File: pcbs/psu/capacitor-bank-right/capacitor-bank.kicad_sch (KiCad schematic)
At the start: 19 parts, among them J1 Conn_01x03, J2 Conn_01x03

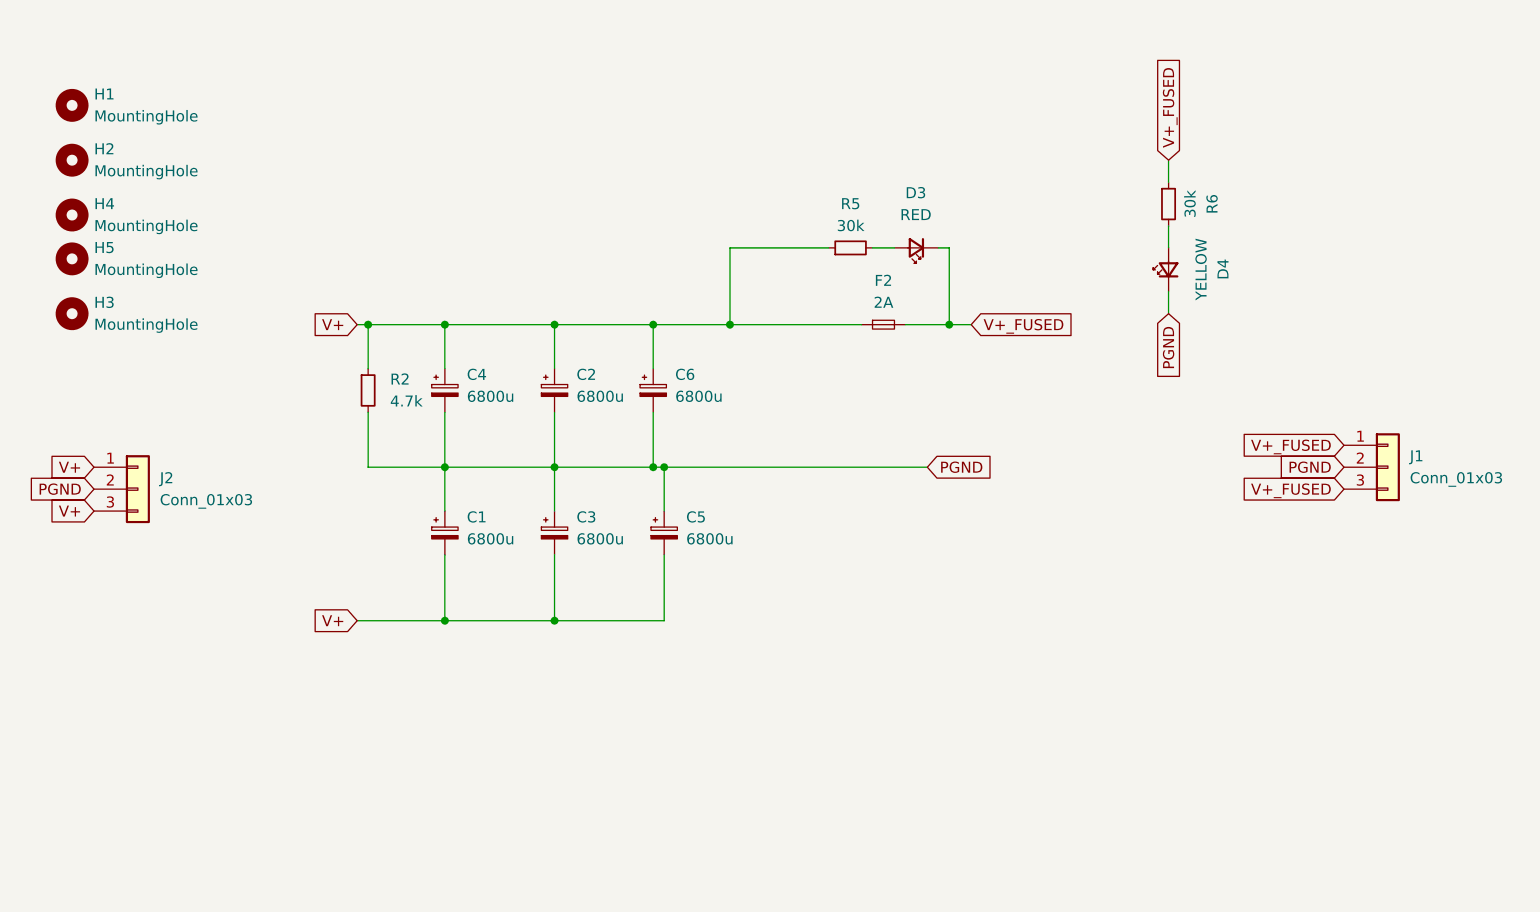
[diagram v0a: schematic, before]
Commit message: All changes
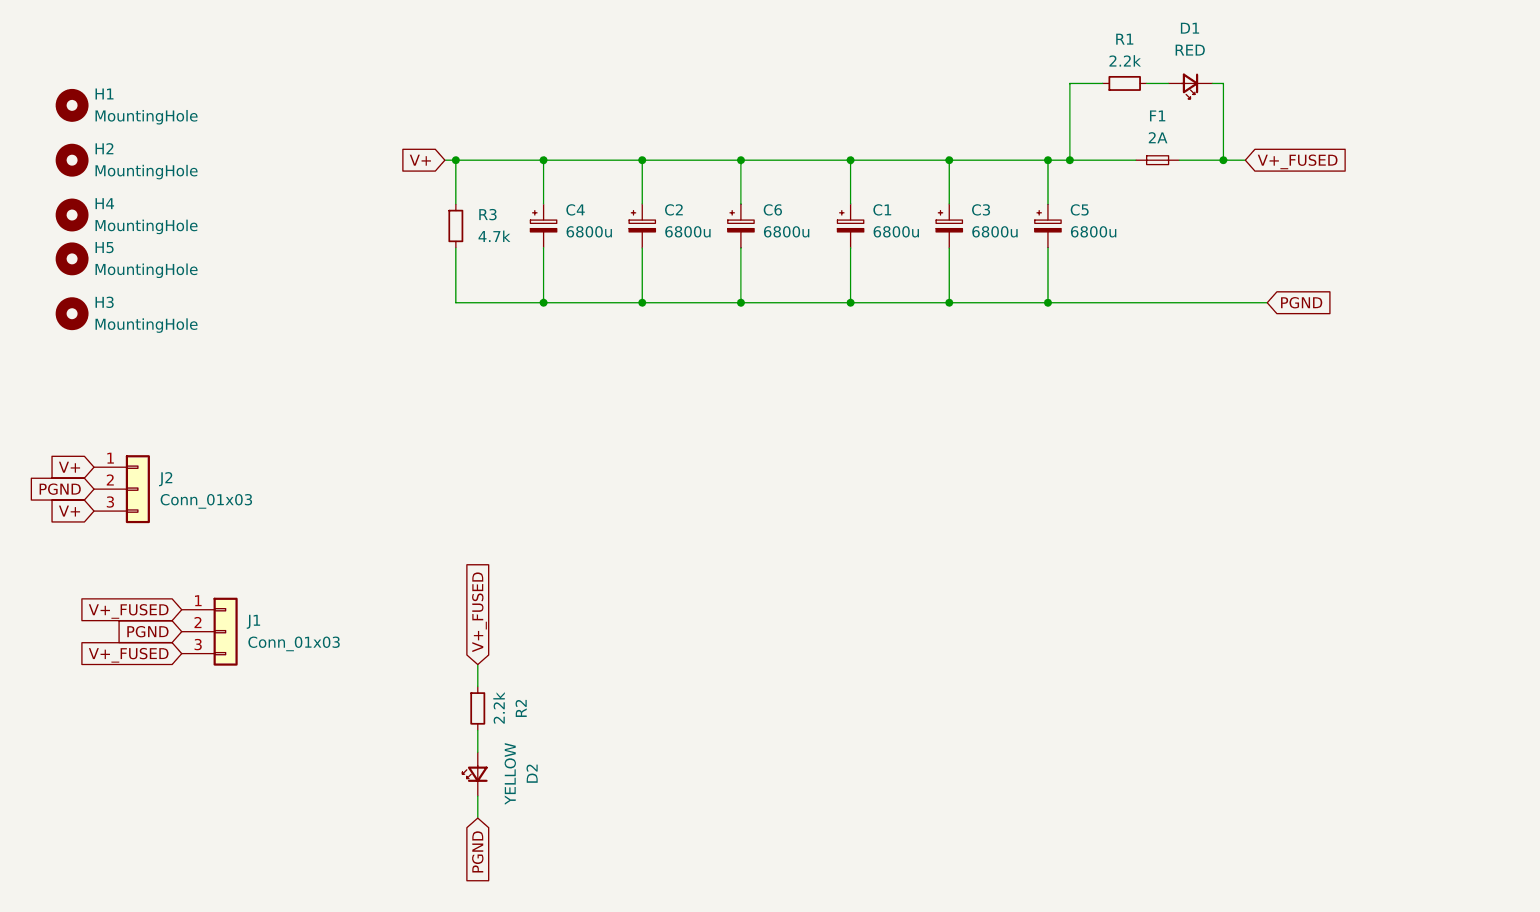
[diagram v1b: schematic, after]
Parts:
- R1: renamed from R5; value 30k -> 2.2k
- R2: renamed from R6; value 30k -> 2.2k
- renumbered D3 to D1, D4 to D2, F2 to F1, R2 to R3
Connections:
- net PGND: now also C1.2, C3.2, C5.2; no longer C1.1, C3.1, C5.1
- net V+: now also C1.1, C3.1, C5.1; no longer C1.2, C3.2, C5.2
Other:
- moved on the sheet: C1, C2, C3, C4, C5, C6, D1, D2, F1, J1, R1, R2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
